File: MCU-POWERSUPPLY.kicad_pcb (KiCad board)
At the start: 2 copper layers, 90 x 27.5 mm, 9 parts, among them J3 Barrel_Jack, J4 USB_B_Micro, U4 LM2596S-5

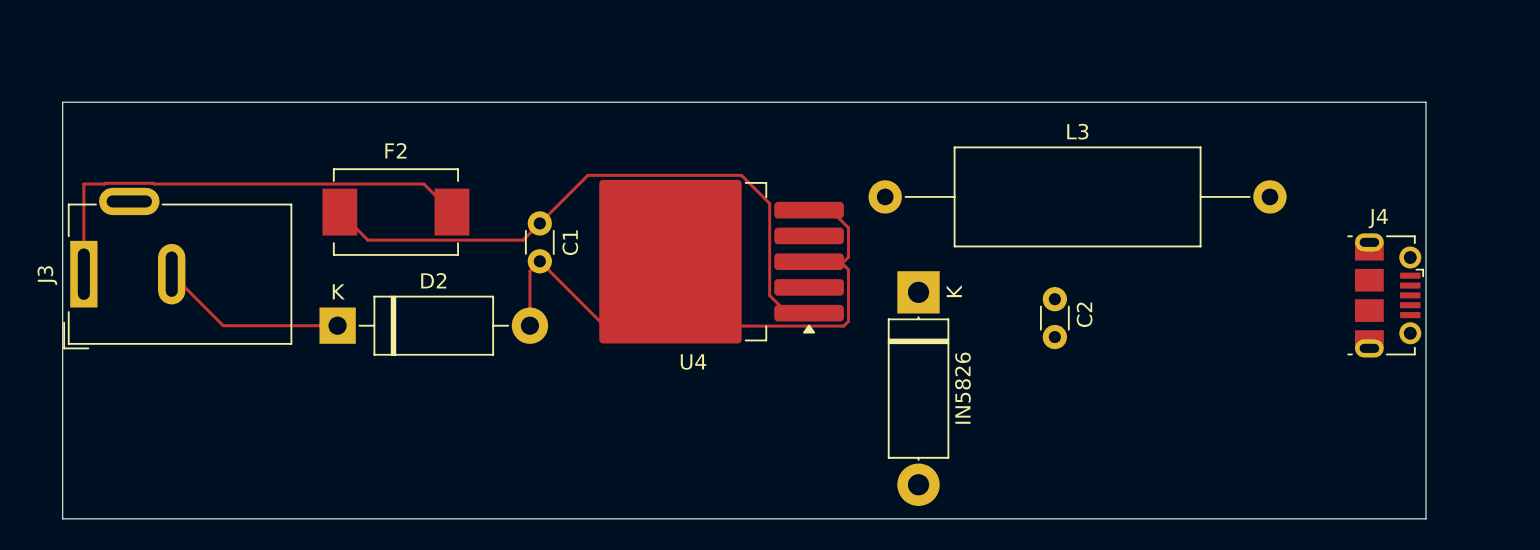
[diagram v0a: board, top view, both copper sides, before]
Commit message: a
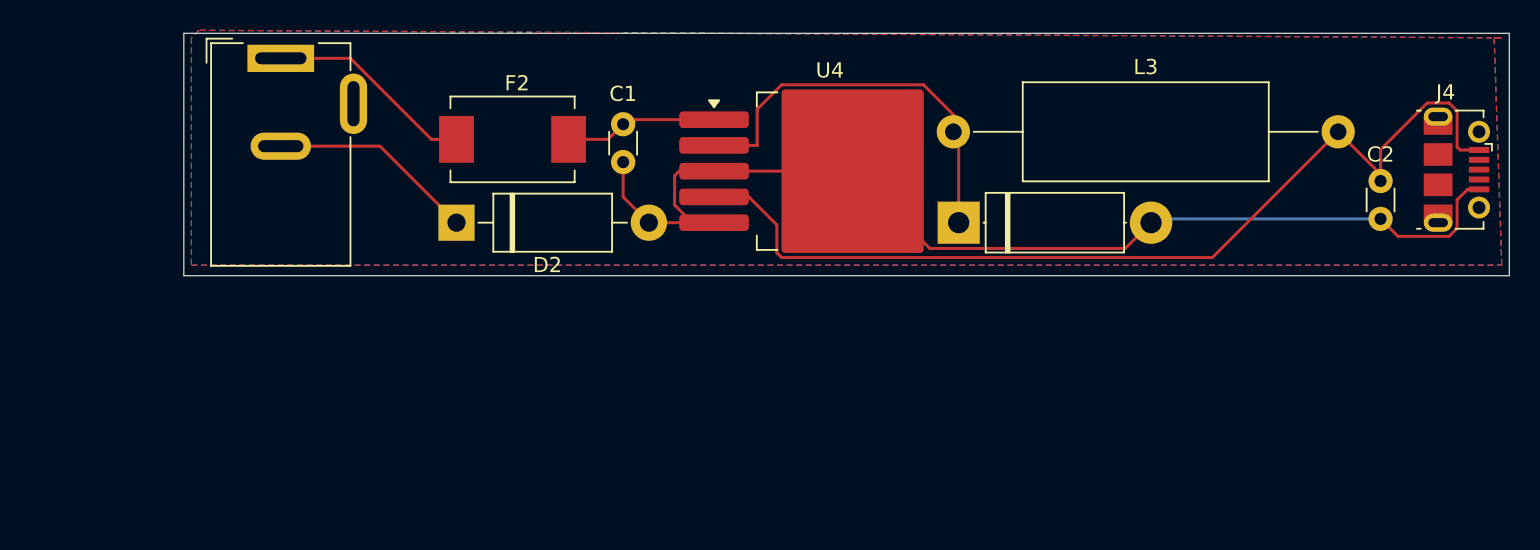
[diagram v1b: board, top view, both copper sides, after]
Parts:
- moved C2 22.9 mm to (151.5, 94.5)
- moved J3 19.3 mm to (78.9, 86.3), turned to 0 degrees
- moved U4 10.8 mm to (115.2, 93.8), turned to 0 degrees
- moved D2 10.4 mm to (90.5, 97.2)
- moved J4 9.46 mm to (156.5, 93.7)
- moved F2 9.07 mm to (94.2, 91.7), turned to 180 degrees
- moved C1 8.55 mm to (101.5, 90.7)
- moved L3 6.22 mm to (123.3, 91.2)
- moved IN5826 5.31 mm to (123.7, 97.2), turned to 0 degrees
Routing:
- net +5V: track 0.25 -> 64.3 mm
- net GND: track 41.2 -> 73.0 mm
- net +12V: track 40.8 -> 10.1 mm
- net Net-(IN5826-K): track 0.00 -> 27.0 mm
- net Net-(F2-Pad2): track 31.1 -> 13.8 mm
- net Net-(D2-K): track 12.4 -> 13.7 mm
- added copper zone on B.Cu, net GND
- added copper zone on F.Cu, net GND
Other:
- board size 90 x 27.5 mm -> 87.5 x 16 mm
